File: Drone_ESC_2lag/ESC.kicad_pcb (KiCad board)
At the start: 2 copper layers, 71.8 x 126.2 mm, 103 parts, among them IC1 STSPIN32G4, J2 Conn_01x02_Pin, J3 Conn_01x02_Pin, J4 Conn_01x03_Pin, P1 USB_C_Plug_USB2.0, Q1 STL130N6F7, Q2 STL130N6F7, Q3 STL130N6F7, Q4 STL130N6F7, Q5 STL130N6F7, Q6 STL130N6F7, SW1 JS102011SAQN, Y1 24.000MHz

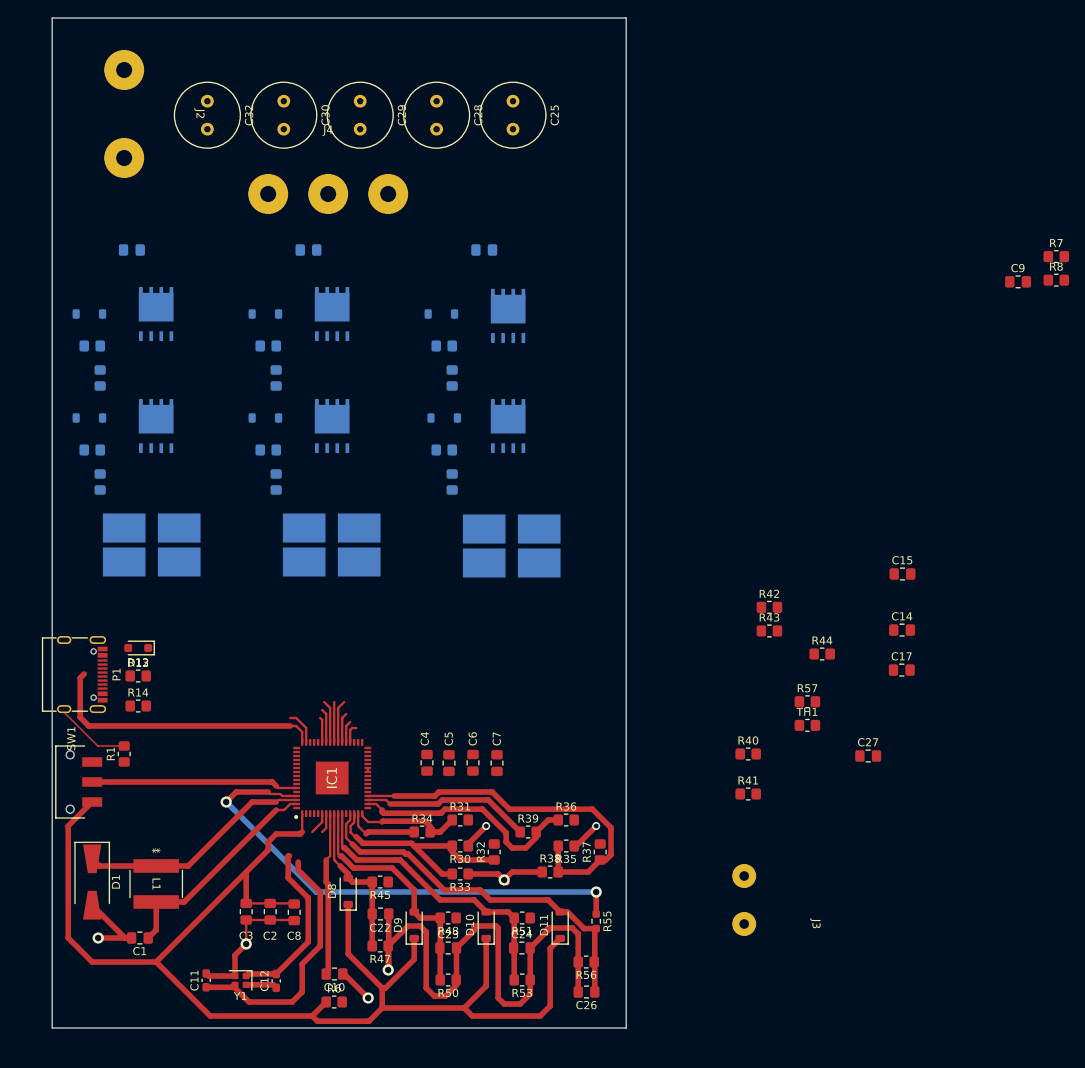
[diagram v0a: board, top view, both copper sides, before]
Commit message: Færdig PCB burde det være
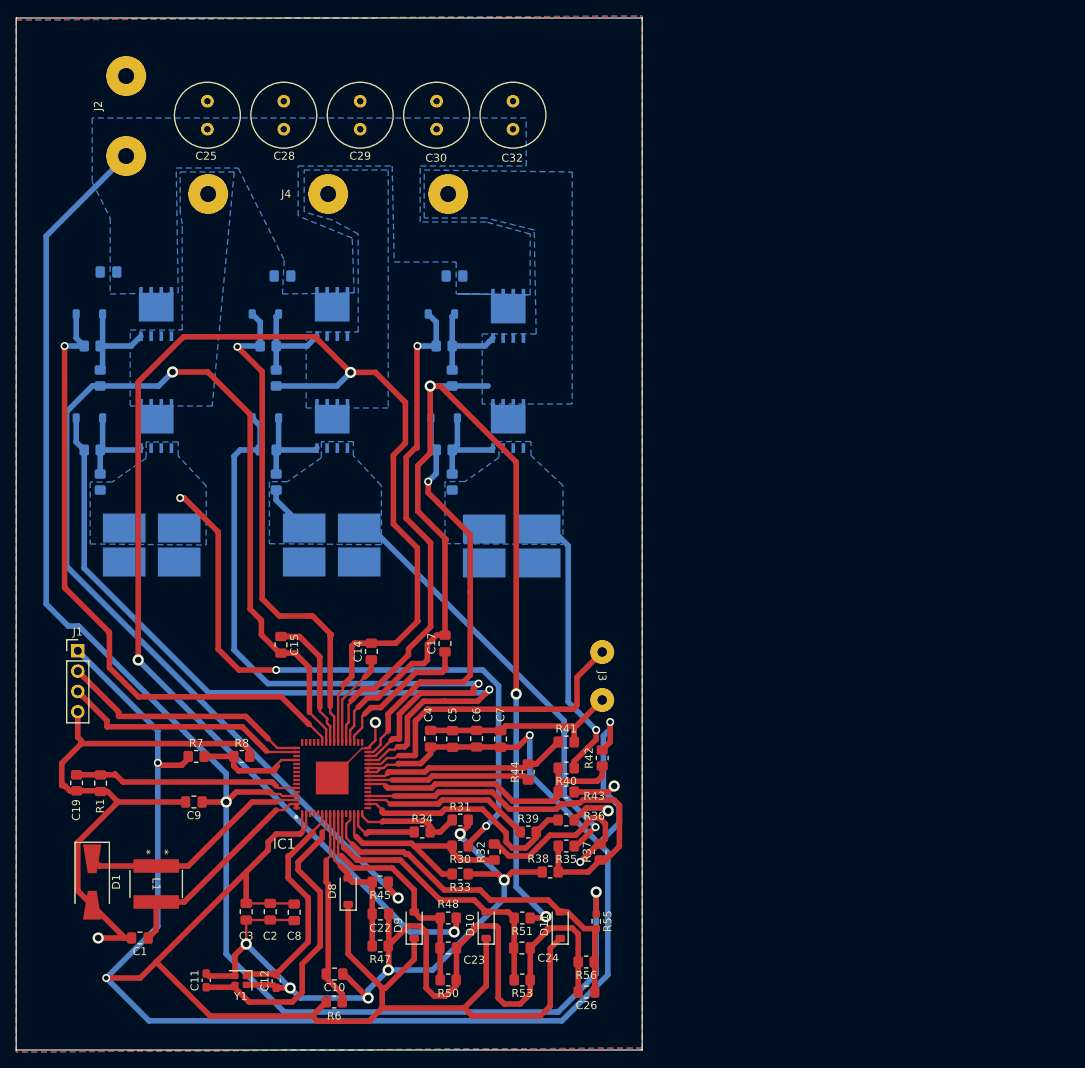
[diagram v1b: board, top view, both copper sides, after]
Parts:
- removed C27: 33nF, Capacitor_SMD:C_0805_2012Metric_Pad1.18x1.45mm_HandSolder
- removed D12: PMEG45T10EXD-QX, Diode_SMD:D_SOD-323_HandSoldering
- removed P1: USB_C_Plug_USB2.0, Connector_USB:USB_C_Receptacle_G-Switch_GT-USB-7010ASV
- removed R13, R14: 5.1k, Resistor_SMD:R_0805_2012Metric_Pad1.20x1.40mm_HandSolder
- removed R57: 4.7k, Resistor_SMD:R_0805_2012Metric_Pad1.20x1.40mm_HandSolder
- removed SW1: JS102011SAQN, Switch:SW_JS102011SAQN
- removed TH1: Thermistor_NTC, Resistor_SMD:R_0805_2012Metric_Pad1.20x1.40mm_HandSolder
- added C19: 100nF, Capacitor_SMD:C_0805_2012Metric_Pad1.18x1.45mm_HandSolder, F.Cu at (41.0, 120.7)
- added J1: Conn_01x04, Connector_PinHeader_2.54mm:PinHeader_1x04_P2.54mm_Vertical, F.Cu at (38.2, 104.1)
- moved R7 124.3 mm to (53.0, 117.3)
- moved C9 121.8 mm to (52.7, 123.0), turned to 180 degrees
- moved R8 117.9 mm to (58.7, 117.3)
- moved C15 78.2 mm to (63.6, 103.3), turned to -90 degrees
- moved C14 66.4 mm to (74.9, 104.2), turned to 90 degrees
- moved C17 57.2 mm to (84.1, 103.2), turned to 90 degrees
- moved R44 39.6 mm to (94.5, 119.2), turned to 90 degrees
- moved C25 38.4 mm to (54.4, 38.9), turned to 90 degrees
- moved C32 38.4 mm to (92.6, 38.9), turned to 90 degrees
- moved J3 33.2 mm to (112.2, 110.2)
- moved R43 32.4 mm to (99.2, 121.8), turned to 180 degrees
- moved R42 28.1 mm to (103.8, 117.5), turned to 90 degrees
- moved R41 23.7 mm to (99.2, 115.5)
- moved R40 22.8 mm to (99.2, 118.8), turned to 180 degrees
- moved C28 19.4 mm to (64.0, 38.9), turned to 90 degrees
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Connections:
- IC1 pad 21: PC4 -> unconnected-(IC1-PC4-Pad21)
- IC1 pad 47: USB_D- -> unconnected-(IC1-PA11-Pad47)
- IC1 pad 48: USB_D+ -> unconnected-(IC1-PA12-Pad48)
- IC1 pad 49: unconnected-(IC1-PA13-Pad49) -> PA13
- IC1 pad 50: unconnected-(IC1-PA14-Pad50) -> PA14
- R1 pad 1: Net-(SW1-C) -> Net-(IC1-PB8)
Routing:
- net VDD: track 166.8 -> 371.6 mm, vias 0 -> 5
- net PHASE_V: track 5.36 -> 190.9 mm, vias 0 -> 3
- net GND: track 130.0 -> 281.9 mm, vias 5 -> 10
- net PHASE_U: track 4.26 -> 153.7 mm, vias 0 -> 2
- net PHASE_W: track 2.40 -> 136.2 mm, vias 0 -> 3
- net VM: track 63.2 -> 191.1 mm
- net GLS1: track 0.00 -> 97.3 mm, vias 0 -> 1
- net GLS2: track 0.00 -> 84.2 mm, vias 0 -> 1
- net VSHUNT1P: track 3.43 -> 80.6 mm, vias 1 -> 3
- net GHS1: track 3.15 -> 80.2 mm, vias 0 -> 1
- net GHS3: track 2.76 -> 63.5 mm, vias 0 -> 1
- net GHS2: track 5.05 -> 64.3 mm, vias 0 -> 1
- net VSHUNT2P: track 3.79 -> 60.4 mm
- net GLS3: track 0.00 -> 53.5 mm, vias 0 -> 1
- net PB10: track 0.00 -> 39.6 mm
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- added copper zone on B.Cu, net GND
- added copper zone on F.Cu, net GND
- added copper zone on B.Cu, net PHASE_U
- added copper zone on B.Cu, net PHASE_V
- added copper zone on B.Cu, net PHASE_W
- added copper zone on B.Cu, net VM
- added copper zone on B.Cu, net VSHUNT1P
- added copper zone on B.Cu, net VSHUNT2P
- added copper zone on B.Cu, net VSHUNT3P
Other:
- board size 71.8 x 126.2 mm -> 78.2 x 129 mm
